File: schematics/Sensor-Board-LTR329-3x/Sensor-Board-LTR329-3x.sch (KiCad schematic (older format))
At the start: 10 parts, among them P1 CONN_02X04, U1 LTR-329ALS-01, U2 LTR-329ALS-01, U3 LTR-329ALS-01

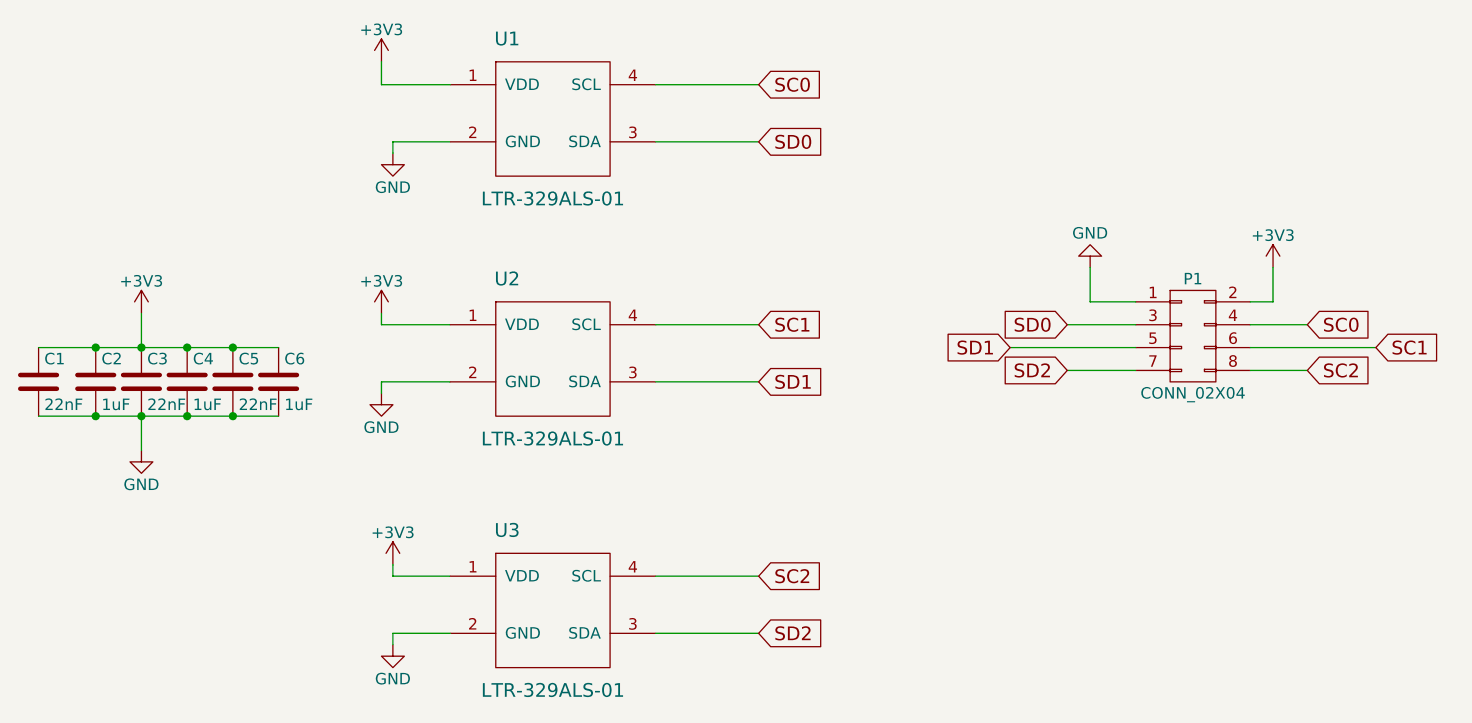
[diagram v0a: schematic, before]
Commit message: Schematics update
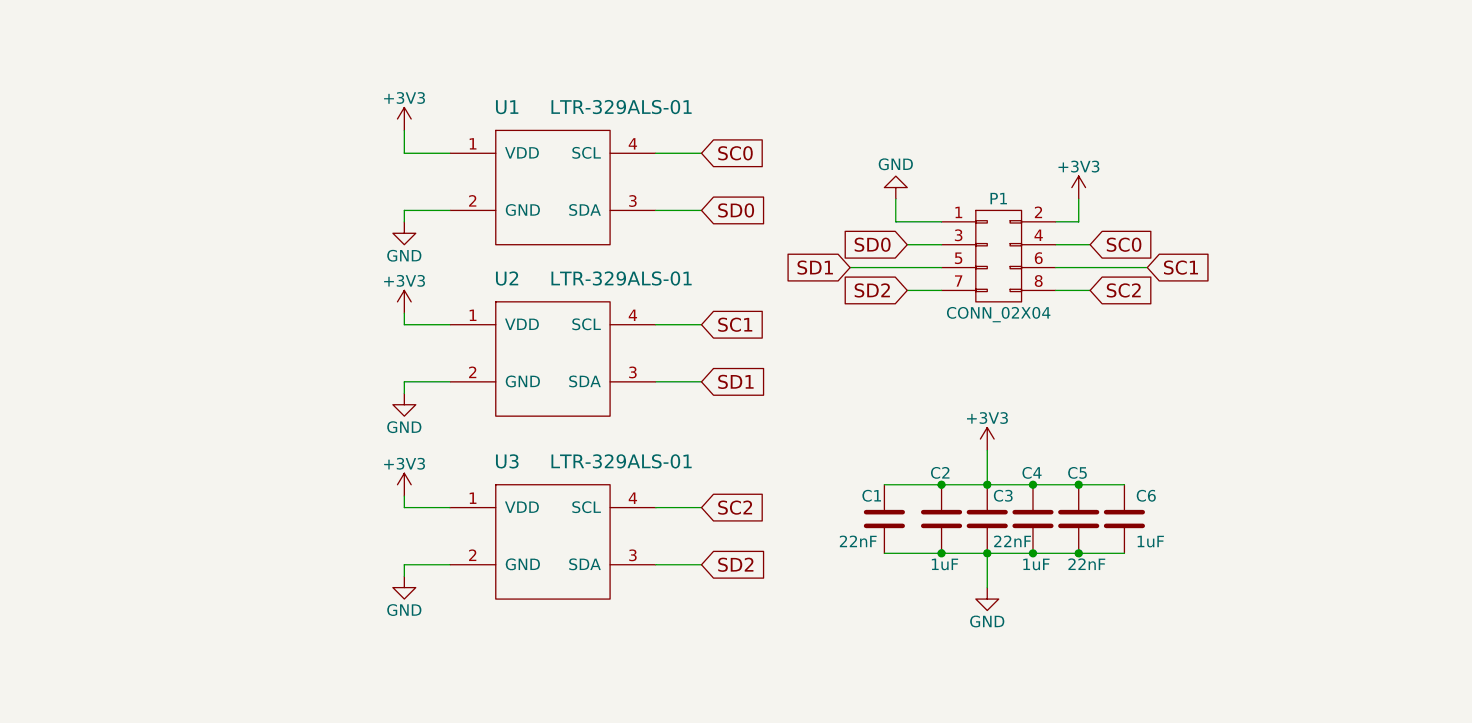
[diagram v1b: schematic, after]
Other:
- moved on the sheet: C1, C2, C3, C4, C5, C6, P1, U1, U3
